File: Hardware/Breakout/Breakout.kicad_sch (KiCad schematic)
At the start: 1 part, among them IC1 NUCLEO-G431KB

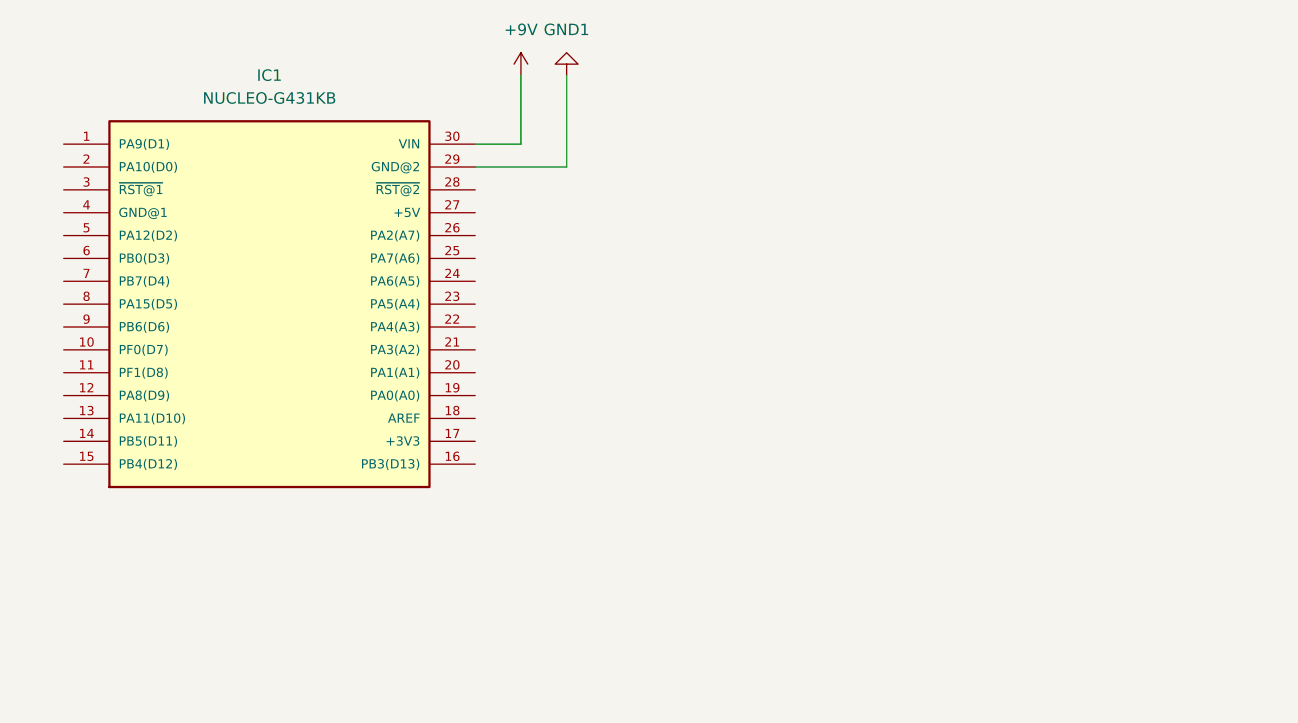
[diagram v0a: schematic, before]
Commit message: Added few parts
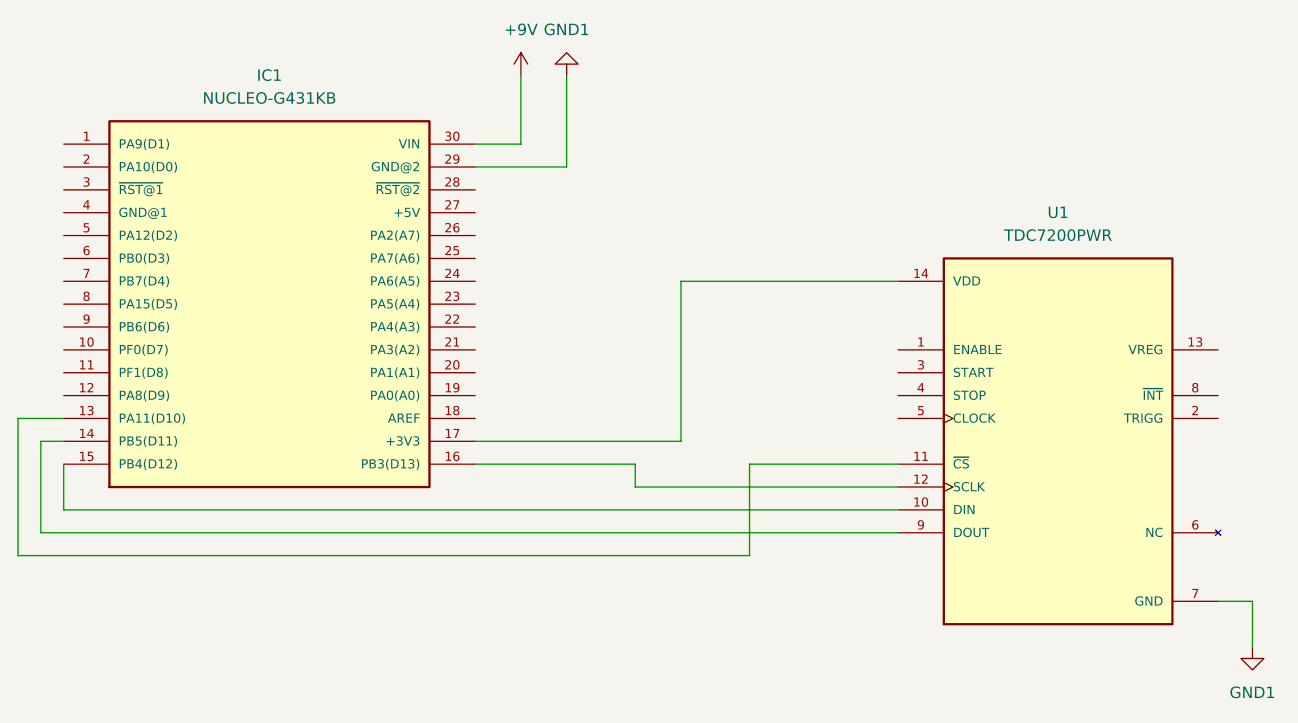
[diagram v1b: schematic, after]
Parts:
- added U1: TDC7200PWR, SOP65P640X120-14N, symbol TDC7200PWR:TDC7200PWR
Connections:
- net GND1: now also U1.7 (GND)
- net at IC1.13 (PA11(D10)): now also U1.11 (~{CS})
- net at IC1.14 (PB5(D11)): now also U1.9 (DOUT)
- net at IC1.15 (PB4(D12)): now also U1.10 (DIN)
- net at IC1.16 (PB3(D13)): now also U1.12 (SCLK)
- net at IC1.17 (+3V3): now also U1.14 (VDD)
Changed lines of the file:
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@@
+    (stroke (width 0) (type default))
+  )
+  (wire (pts (xy 66.04 101.6) (xy 66.04 116.84))
+    (stroke (width 0) (type default))
+  )
+  (wire (pts (xy 116.84 106.68) (xy 134.62 106.68))
+    (stroke (width 0) (type default))
+  )
+  (wire (pts (xy 147.32 116.84) (xy 147.32 106.68))
+    (stroke (width 0) (type default))
+  )
+  (wire (pts (xy 134.62 109.22) (xy 163.83 109.22))
+    (stroke (width 0) (type default))
+  )
+  (wire (pts (xy 134.62 106.68) (xy 134.62 109.22))
     (stroke (width 0) (type default))
   )
@@
     (stroke (width 0) (type default))
   )
+  (wire (pts (xy 68.58 104.14) (xy 68.58 114.3))
+    (stroke (width 0) (type default))
+  )
+  (wire (pts (xy 68.58 114.3) (xy 163.83 114.3))
+    (stroke (width 0) (type default))
+  )
   (wire (pts (xy 116.84 71.12) (xy 121.92 71.12))
     (stroke (width 0) (type default))
   )
+  (wire (pts (xy 71.12 101.6) (xy 66.04 101.6))
+    (stroke (width 0) (type default))
+  )
+  (wire (pts (xy 147.32 106.68) (xy 163.83 106.68))
+    (stroke (width 0) (type default))
+  )
+  (wire (pts (xy 139.7 86.36) (xy 163.83 86.36))
+    (stroke (width 0) (type default))
+  )
+  (wire (pts (xy 71.12 111.76) (xy 163.83 111.76))
+    (stroke (width 0) (type default))
+  )
+  (wire (pts (xy 116.84 104.14) (xy 139.7 104.14))
+    (stroke (width 0) (type default))
+  )
+  (wire (pts (xy 139.7 104.14) (xy 139.7 86.36))
+    (stroke (width 0) (type default))
+  )
+  (wire (pts (xy 66.04 116.84) (xy 147.32 116.84))
+    (stroke (width 0) (type default))
+  )
+  (wire (pts (xy 71.12 106.68) (xy 71.12 111.76))
+    (stroke (width 0) (type default))
+  )
   (wire (pts (xy 127 73.66) (xy 116.84 73.66))
     (stroke (width 0) (type default))
   )
+  (wire (pts (xy 199.39 121.92) (xy 203.2 121.92))
+    (stroke (width 0) (type default))
+  )
+  (wire (pts (xy 203.2 121.92) (xy 203.2 127))
+    (stroke (width 0) (type default))
+  )
+  (wire (pts (xy 71.12 104.14) (xy 68.58 104.14))
+    (stroke (width 0) (type default))
+  )
   (symbol (lib_id "power:GND1") (at 127 63.5 180) (unit 1)
     (in_bom yes) (on_board yes) (dnp no) (fields_autoplaced)
@@
         (path "/c2ef38f9-0f55-4b19-9130-d81b036a0cd1"
           (reference "#PWR01") (unit 1)
+        )
+      )
+    )
+  )
+  (symbol (lib_id "power:GND1") (at 203.2 127 0) (unit 1)
+    (in_bom yes) (on_board yes) (dnp no) (fields_autoplaced)
+    (property "Reference" "#PWR03" (at 203.2 133.35 0)
+      (effects (font (size 1.27 1.27)) hide)
+    )
+    (property "Value" "GND1" (at 203.2 132.08 0)
+      (effects (font (size 1.27 1.27)))
+    )
+    (property "Footprint" "" (at 203.2 127 0)
+      (effects (font (size 1.27 1.27)) hide)
+    )
+    (property "Datasheet" "" (at 203.2 127 0)
+      (effects (font (size 1.27 1.27)) hide)
+    )
+    (pin "1")
+    (instances
+      (project "Breakout"
+        (path "/c2ef38f9-0f55-4b19-9130-d81b036a0cd1"
+          (reference "#PWR03") (unit 1)
         )
       )
@@
         )
       )
+    )
+  )
+  (symbol (lib_id "TDC7200PWR:TDC7200PWR") (at 181.61 104.14 0) (unit 1)
+    (in_bom yes) (on_board yes) (dnp no) (fields_autoplaced)
+    (property "Reference" "U1" (at 181.61 78.74 0)
+      (effects (font (size 1.27 1.27)))
+    )
+    (property "Value" "TDC7200PWR" (at 181.61 81.28 0)
+      (effects (font (size 1.27 1.27)))
+    )
+    (property "Footprint" "SOP65P640X120-14N" (at 181.61 104.14 0)
+      (effects (font (size 1.27 1.27)) (justify bottom) hide)
+    )
+    (property "Datasheet" "" (at 181.61 104.14 0)
+      (effects (font (size 1.27 1.27)) hide)
+    )
+    (property "PARTREV" "D" (at 181.61 104.14 0)
+      (effects (font (size 1.27 1.27)) (justify bottom) hide)
+    )
+    (property "MANUFACTURER" "Texas Instruments" (at 181.61 104.14 0)
+      (effects (font (size 1.27 1.27)) (justify bottom) hide)
+    )
+    (property "MAXIMUM_PACKAGE_HEIGHT" "1.2 mm" (at 181.61 104.14 0)
+      (effects (font (size 1.27 1.27)) (justify bottom) hide)
+    )
+    (property "STANDARD" "IPC 7351B" (at 181.61 104.14 0)
+      (effects (font (size 1.27 1.27)) (justify bottom) hide)
+    )
+    (pin "1")
+    (pin "10")
+    (pin "11")
+    (pin "12")
+    (pin "13")
+    (pin "14")
+    (pin "2")
+    (pin "3")
+    (pin "4")
+    (pin "5")
+    (pin "6")
+    (pin "7")
+    (pin "8")
+    (pin "9")
+    (instances
+      (project "Breakout"
+        (path "/c2ef38f9-0f55-4b19-9130-d81b036a0cd1"
+          (reference "U1") (unit 1)
+        )
+      )
